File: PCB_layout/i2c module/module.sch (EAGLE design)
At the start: 7 parts, among them IC1 ATTINY85-20SU, J1 M20-9980346

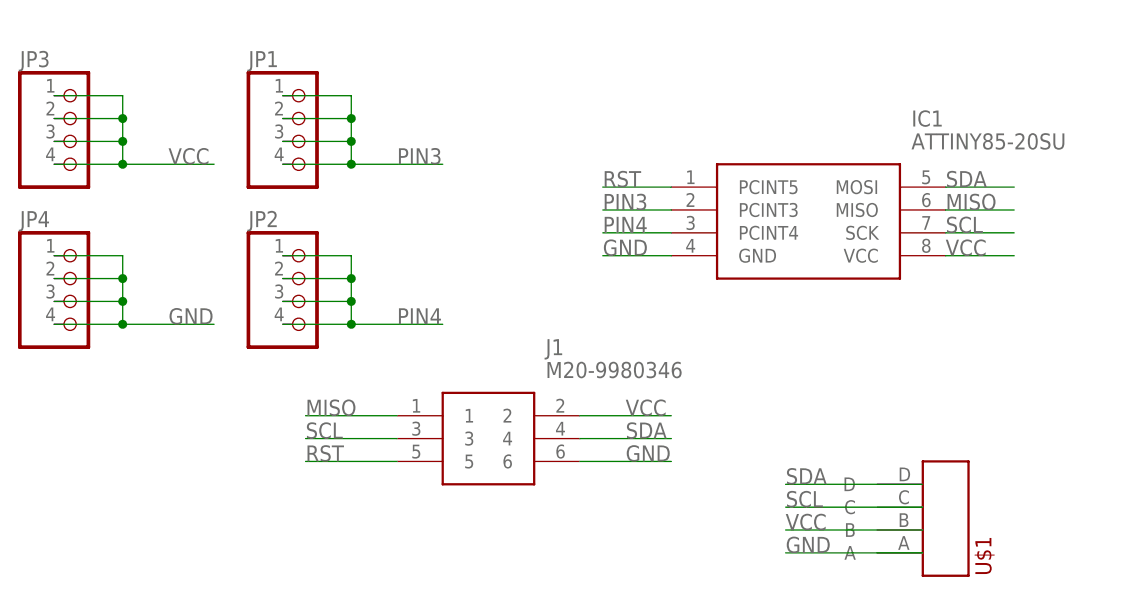
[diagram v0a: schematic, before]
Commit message: reorg, i2c dev, lbr updates
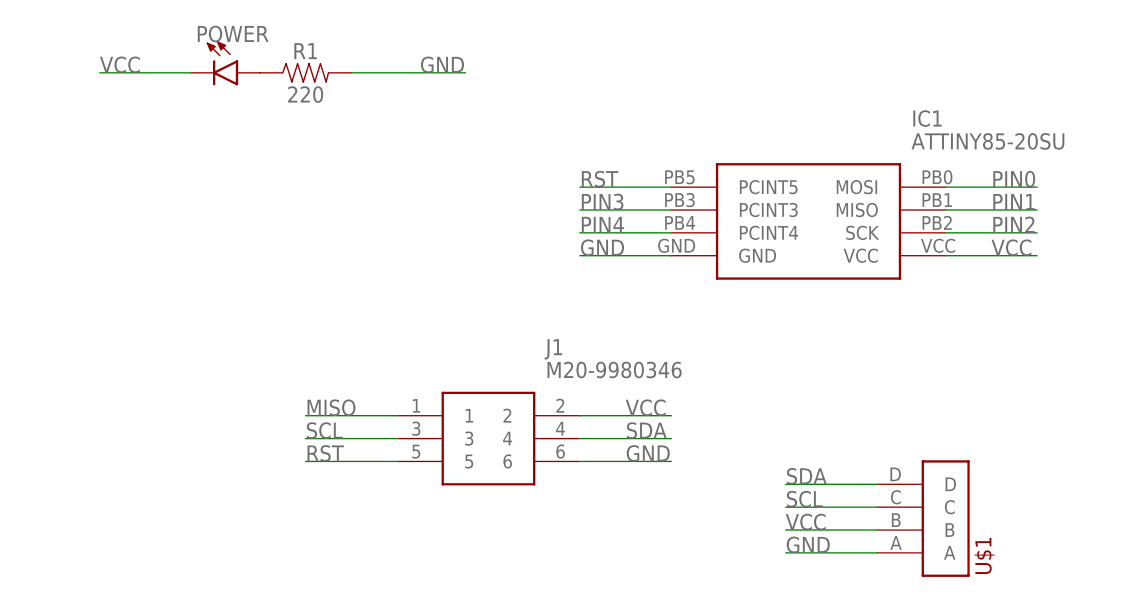
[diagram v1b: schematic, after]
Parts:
- removed JP1, JP2, JP3, JP4: (no value), pinhead:PINHD-1X4
- added POWER: (no value), SparkFun-LED:LED3MM
- added R1: 220, SparkFun-Resistors:RESISTORAXIAL-0.3
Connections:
- new net N$11: POWER.A, R1.1
- new net PIN0: IC1.MOSI
- new net PIN1: IC1.MISO
- new net PIN2: IC1.SCK
- net GND: now also R1.2; no longer JP4.1, JP4.2, JP4.3, JP4.4
- net MISO: no longer IC1.MISO
- net PIN3: no longer JP1.1, JP1.2, JP1.3, JP1.4
- net PIN4: no longer JP2.1, JP2.2, JP2.3, JP2.4
- net SCL: no longer IC1.SCK
- net SDA: no longer IC1.MOSI
- net VCC: now also POWER.C; no longer JP3.1, JP3.2, JP3.3, JP3.4
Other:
- moved on the sheet: U$1
